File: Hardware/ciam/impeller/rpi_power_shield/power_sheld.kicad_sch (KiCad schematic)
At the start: 18 parts, among them J1 PLS-3, SW1 KLS7-TS6601-11-180, U1 STM32F401RCTx, Y1 KSE-7K32768KDY2400A3

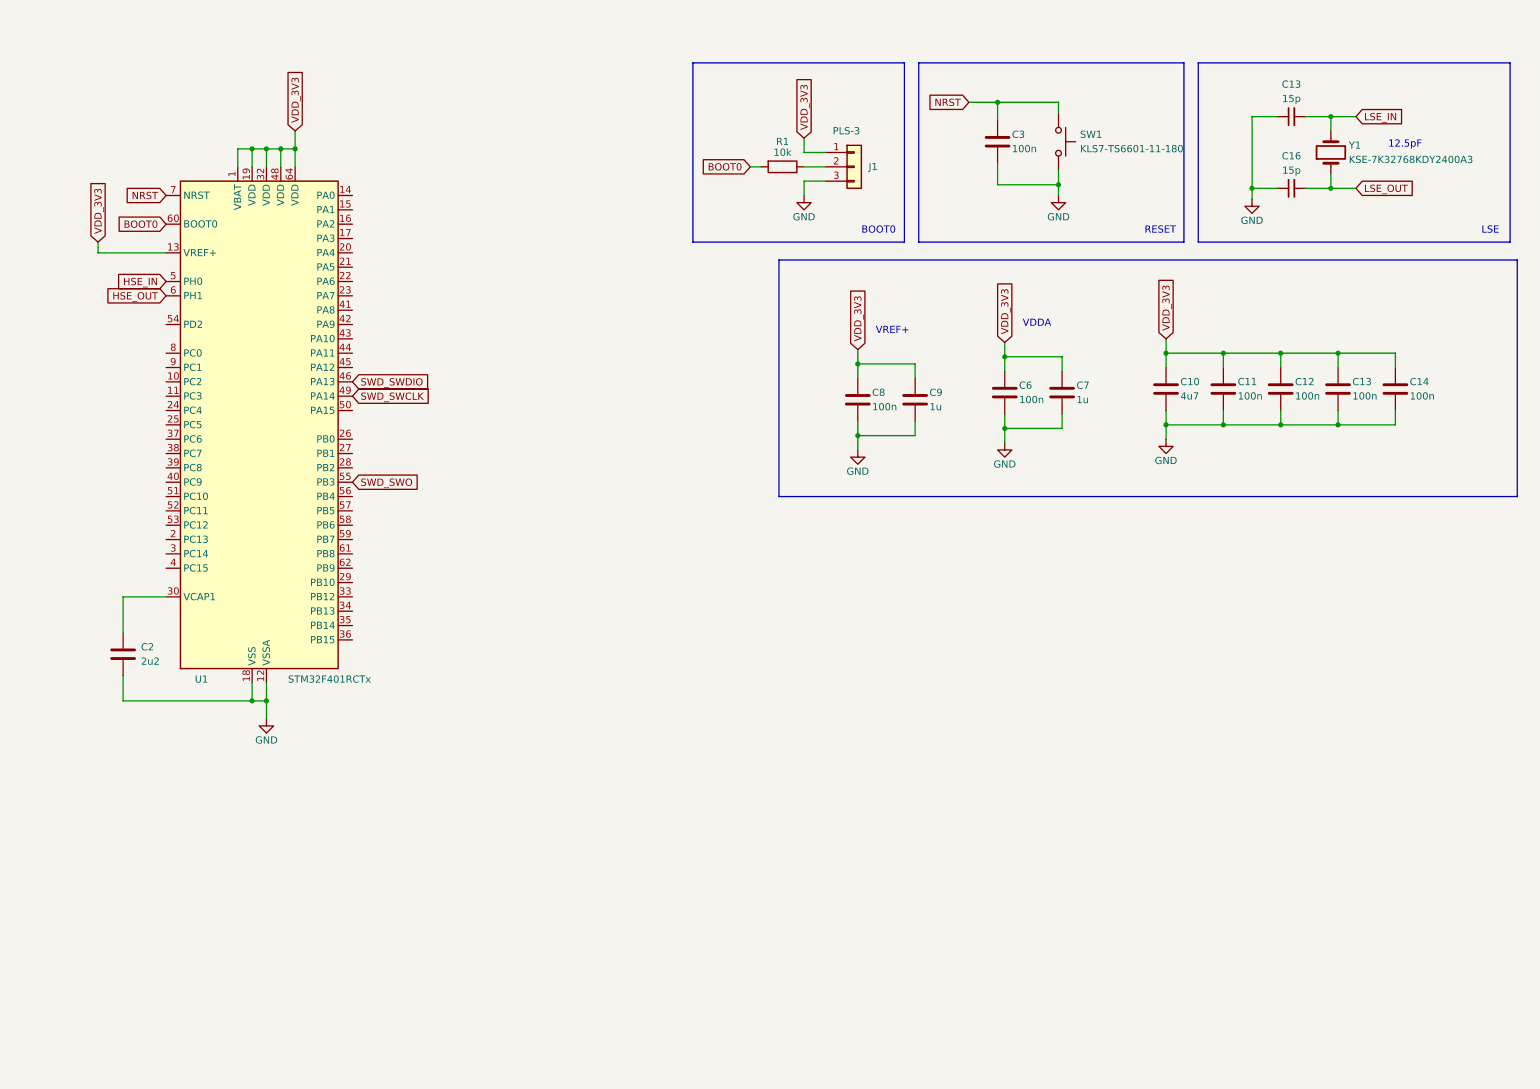
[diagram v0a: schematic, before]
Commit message: added rpi shield project
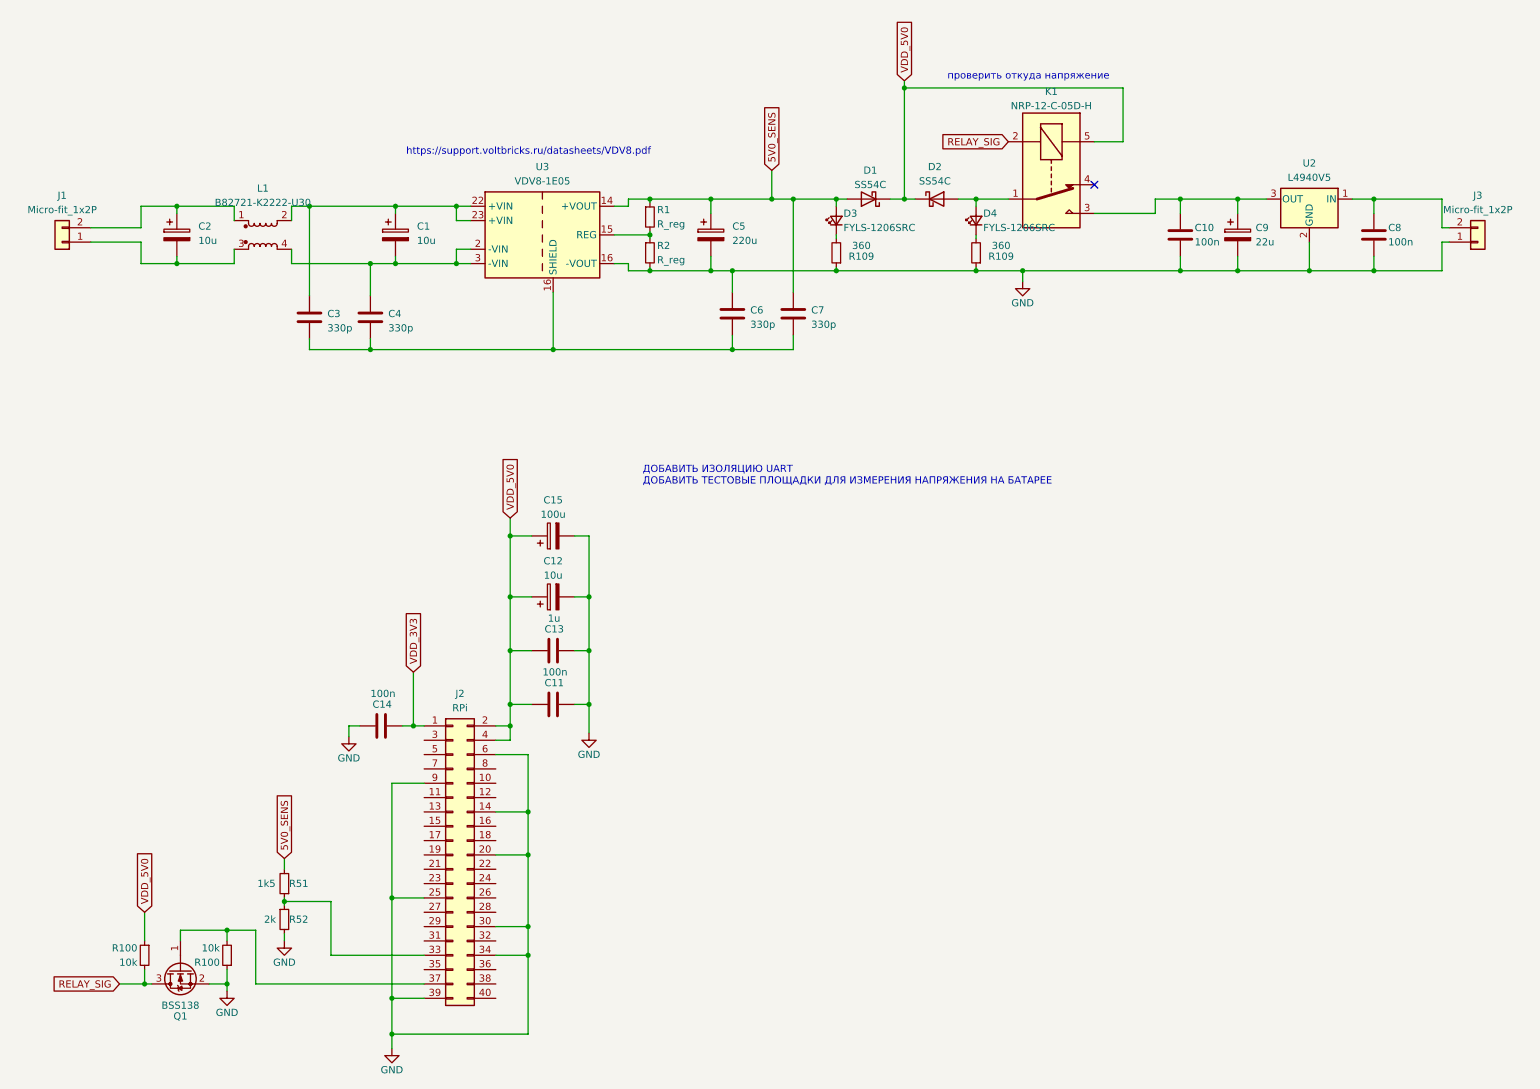
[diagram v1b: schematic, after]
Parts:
- removed C12: 100n, Capacitor_SMD:C_0603_1608Metric, symbol Device:C
- removed C13, C16: 15p, Capacitor_SMD:C_0603_1608Metric, symbol Device:C_Small
- removed C2: 2u2, Capacitor_SMD:C_0603_1608Metric, symbol Device:C
- removed C9: 1u, Capacitor_SMD:C_0603_1608Metric, symbol Device:C
- removed J1: PLS-3, Connector_PinHeader_2.54mm:PinHeader_1x03_P2.54mm_Vertical, symbol Connector_Generic:Conn_01x03
- removed R1: 10k, Resistor_SMD:R_0805_2012Metric, symbol Device:R
- removed SW1: KLS7-TS6601-11-180, Button_Switch_THT:SW_PUSH_6mm_H4.3mm, symbol Switch:SW_Push
- removed U1: STM32F401RCTx, Package_QFP:LQFP-64_10x10mm_P0.5mm, symbol MCU_ST_STM32F4:STM32F401RCTx
- removed Y1: KSE-7K32768KDY2400A3, user_lib:KSE-7K32768KDY2400A3, symbol Device:Crystal
- added C1, C12, C2: 10u, symbol Device:C_Polarized
- added C15: 100u, symbol Device:C_Polarized
- added C4: 330p, symbol Device:C
- added C5: 220u, symbol Device:C_Polarized
- added C9: 22u, symbol Device:C_Polarized
- added D1, D2: SS54C, symbol Device:D_Schottky
- added D3, D4: FYLS-1206SRC, Resistor_SMD:R_1206_3216Metric_Pad1.30x1.75mm_HandSolder, symbol Device:LED_Small
- added J1, J3: Micro-fit_1x2P, symbol Connector_Generic:Conn_01x02
- added J2: RPi, symbol Connector_Generic:Conn_02x20_Odd_Even
- added K1: NRP-12-C-05D-H, symbol Relay:SANYOU_SRD_Form_C
- added L1: B82721-K2222-U30, symbol Device:L_Coupled
- added Q1: BSS138, Package_TO_SOT_SMD:SOT-23, symbol Transistor_FET:BSS138
- added R1, R2: R_reg, Resistor_SMD:R_0603_1608Metric, symbol Device:R_Small
- added R100 (x2): 10k, Resistor_SMD:R_0805_2012Metric, symbol Device:R_Small
- added R109 (x2): 360, Resistor_SMD:R_0603_1608Metric, symbol Device:R_Small
- added R51: 1k5, Resistor_SMD:R_0603_1608Metric, symbol Device:R_Small
- added R52: 2k, Resistor_SMD:R_0603_1608Metric, symbol Device:R_Small
- added U2: L4940V5, symbol Regulator_Linear:L7805
- added U3: VDV8-1E05, symbol Converter_DCDC:TMR-1211
- C10: value 4u7 -> 100n; footprint Capacitor_SMD:C_0603_1608Metric -> (none); Ссылка https://www.chipdip.ru/product0/9000348448 -> https://www.chipdip.ru/product/grm319r71h104k; Цена 21 -> 13; Человекопонятное название Конденсатор 4.7мкФ -> Конденсатор керамический
- C11, C14, C8: footprint Capacitor_SMD:C_0603_1608Metric -> (none); Ссылка https://www.chipdip.ru/product/grm188r71h104k -> https://www.chipdip.ru/product/grm319r71h104k; Цена 19 -> 13; Человекопонятное название Конденсатор 100нФ -> Конденсатор керамический
- C13: value 100n -> 1u; footprint Capacitor_SMD:C_0603_1608Metric -> (none); Ссылка https://www.chipdip.ru/product/grm188r71h104k -> https://www.chipdip.ru/product/grm31mr71e105k; Цена 19 -> 25; Человекопонятное название Конденсатор 100нФ -> Конденсатор керамический
- C3, C6: value 100n -> 330p; footprint Capacitor_SMD:C_0603_1608Metric -> (none); Ссылка https://www.chipdip.ru/product/grm188r71h104k -> https://www.chipdip.ru/product/grm31a7u2j331jw31d; Цена 19 -> 25; Человекопонятное название Конденсатор 100нФ -> Керамический конденсатор
- C7: value 1u -> 330p; footprint Capacitor_SMD:C_0603_1608Metric -> (none); Ссылка https://www.chipdip.ru/product/grm188r71c105ka12d -> https://www.chipdip.ru/product/grm31a7u2j331jw31d; Цена 20 -> 25; Человекопонятное название Конденсатор 1мкФ -> Керамический конденсатор
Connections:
- net GND: now also C14.1, C6.1, C12.2, C15.2, C5.2, C9.2, J2.14 (Pin_14), J2.20 (Pin_20), J2.25 (Pin_25), J2.30 (Pin_30), J2.34 (Pin_34), J2.39 (Pin_39), J2.6 (Pin_6), J2.9 (Pin_9), J3.1 (Pin_1), Q1.2 (S), R100.1, R109.1, R109.1, R2.2, R52.2, U2.2 (GND), U3.16 (SHIELD); no longer C14.2, C3.2, C6.2, C7.2
- net VDD_3V3: now also C14.2, J2.1 (Pin_1); no longer C10.1, C11.1, C13.1, C14.1, C6.1, C7.1, C8.1
- net NRST: no longer names the net of C3.1
- net NRST: now also C1.1, L1.2, U3.22 (+VIN), U3.23 (+VIN)
- new net: D4.1 (K), R109.2
- new net: D2.2 (A), D4.2 (A), K1.1
- new net: J2.37 (Pin_37), Q1.1 (G), R100.2
- new net: J2.33 (Pin_33), R51.1, R52.1
- new net: C8.1, J3.2 (Pin_2), U2.1 (IN)
- new net: C10.1, C9.1, K1.3, U2.3 (OUT)
- new net: C2.1, J1.2 (Pin_2), L1.1
- new net: C2.2, J1.1 (Pin_1), L1.3
- new net: C1.2, C4.1, L1.4, U3.2 (-VIN), U3.3 (-VIN)
- new net: D3.1 (K), R109.2
- new net: C3.2, C4.2, C6.2, C7.2, U3.16 (SHIELD)
- new net: R1.2, R2.1, U3.15 (REG)
- new net 5V0_SENS: C5.1, C7.1, D1.2 (A), D3.2 (A), R1.1, R51.2, U3.14 (+VOUT)
- new net RELAY_SIG: K1.2, Q1.3 (D), R100.2
- new net VDD_5V0: C11.1, C12.1, C13.1, C15.1, D1.1 (K), D2.1 (K), J2.2 (Pin_2), J2.4 (Pin_4), K1.5, R100.1
- no-connect marks 0 -> 1
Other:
- note added: "https://support.voltbricks.ru/datasheets/VDV8.pdf"
- note added: "ДОБАВИТЬ ИЗОЛЯЦИЮ UART ДОБАВИТЬ ТЕСТОВЫЕ ПЛОЩАДКИ ДЛЯ ИЗМЕРЕНИЯ НАПРЯЖЕНИЯ НА БАТАРЕЕ"
- note added: "проверить откуда напряжение"
- note removed: "12.5pF"
- note removed: "BOOT0"
- note removed: "LSE"
- note removed: "RESET"
- note removed: "VDDA"
- note removed: "VREF+"

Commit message: added rpi uart isolation
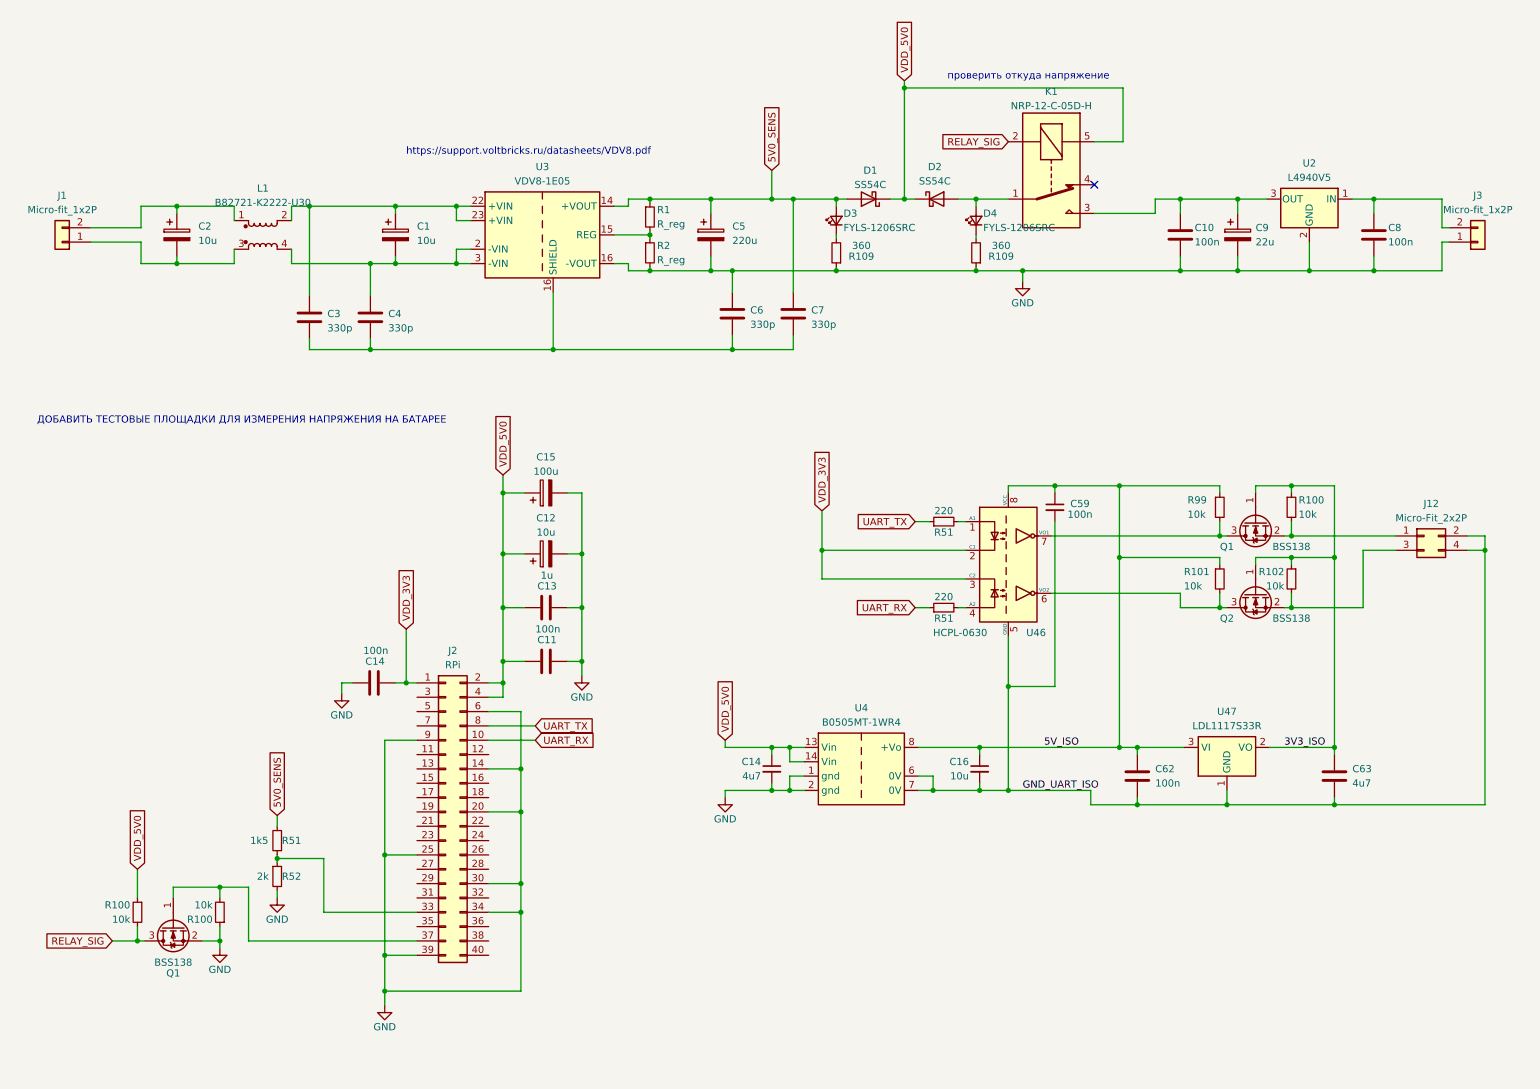
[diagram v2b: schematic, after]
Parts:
- added C14: 4u7, Capacitor_SMD:C_0805_2012Metric, symbol Device:C_Small
- added C16: 10u, Capacitor_SMD:C_0805_2012Metric, symbol Device:C_Small
- added C59: 100n, Capacitor_SMD:C_0805_2012Metric, symbol Device:C_Small
- added C62: 100n, Capacitor_SMD:C_0805_2012Metric, symbol Device:C
- added C63: 4u7, Capacitor_SMD:C_0805_2012Metric, symbol Device:C
- added J12: Micro-Fit_2x2P, Connector_Molex:Molex_Micro-Fit_3.0_43045-0400_2x02_P3.00mm_Horizontal, symbol Connector_Generic:Conn_02x02_Odd_Even
- added Q1, Q2: BSS138, Package_TO_SOT_SMD:SOT-23, symbol Transistor_FET:BSS138
- added R100, R101, R102, R99: 10k, Resistor_SMD:R_0805_2012Metric, symbol Device:R_Small
- added R51 (x2): 220, Resistor_SMD:R_0603_1608Metric, symbol Device:R_Small
- added U4: B0505MT-1WR4, user_lib:B0505MT-1WR4, symbol Interface_CAN_LIN:ISO1050DUB
- added U46: HCPL-0630, Package_SO:SOIC-8_3.9x4.9mm_P1.27mm, symbol Isolator:HCPL-0630
- added U47: LDL1117S33R, Package_TO_SOT_SMD:SOT-223-3_TabPin2, symbol Regulator_Linear:LD1117S33TR_SOT223
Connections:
- net GND: now also C14.2, U4.1 (gnd), U4.2 (gnd)
- net VDD_3V3: now also U46.2 (C1), U46.3 (C2)
- net VDD_5V0: now also C14.1, U4.13 (Vin), U4.14 (Vin)
- net UART_RX: now reaches J2.10 (Pin_10)
- net UART_RX: now also R51.1
- net UART_TX: now reaches J2.8 (Pin_8)
- net UART_TX: now also R51.1
- new net: J12.1 (Pin_1), Q1.2 (S), R100.2
- new net: J12.3 (Pin_3), Q2.2 (S), R102.2
- new net: Q1.3 (D), R99.2, U46.7 (VO1)
- new net: Q2.3 (D), R101.2, U46.6 (VO2)
- new net: R51.2, U46.1 (A1)
- new net: R51.2, U46.4 (A2)
- new net 3V3_ISO: C63.1, Q1.1 (G), Q2.1 (G), R100.1, R102.1, U47.2 (VO)
- new net 5V_ISO: C16.1, C59.1, C62.1, R101.1, R99.1, U4.8 (+Vo), U46.8 (VCC), U47.3 (VI)
- new net GND_UART_ISO: C16.2, C59.2, C62.2, C63.2, J12.2 (Pin_2), J12.4 (Pin_4), U4.6 (0V), U4.7 (0V), U46.5 (GND), U47.1 (GND)
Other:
- note added: "ДОБАВИТЬ ТЕСТОВЫЕ ПЛОЩАДКИ ДЛЯ ИЗМЕРЕНИЯ НАПРЯЖЕНИЯ НА БАТАРЕЕ"
- note removed: "ДОБАВИТЬ ИЗОЛЯЦИЮ UART ДОБАВИТЬ ТЕСТОВЫЕ ПЛОЩАДКИ ДЛЯ ИЗМЕРЕНИЯ НАПРЯЖЕНИЯ НА БАТАРЕЕ"
- moved on the sheet: C11, C12, C13, C14, C15, J2, Q1, R100, R51, R52
